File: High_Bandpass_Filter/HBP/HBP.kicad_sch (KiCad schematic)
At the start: 25 parts, among them IC2 OPA1644AIPWR

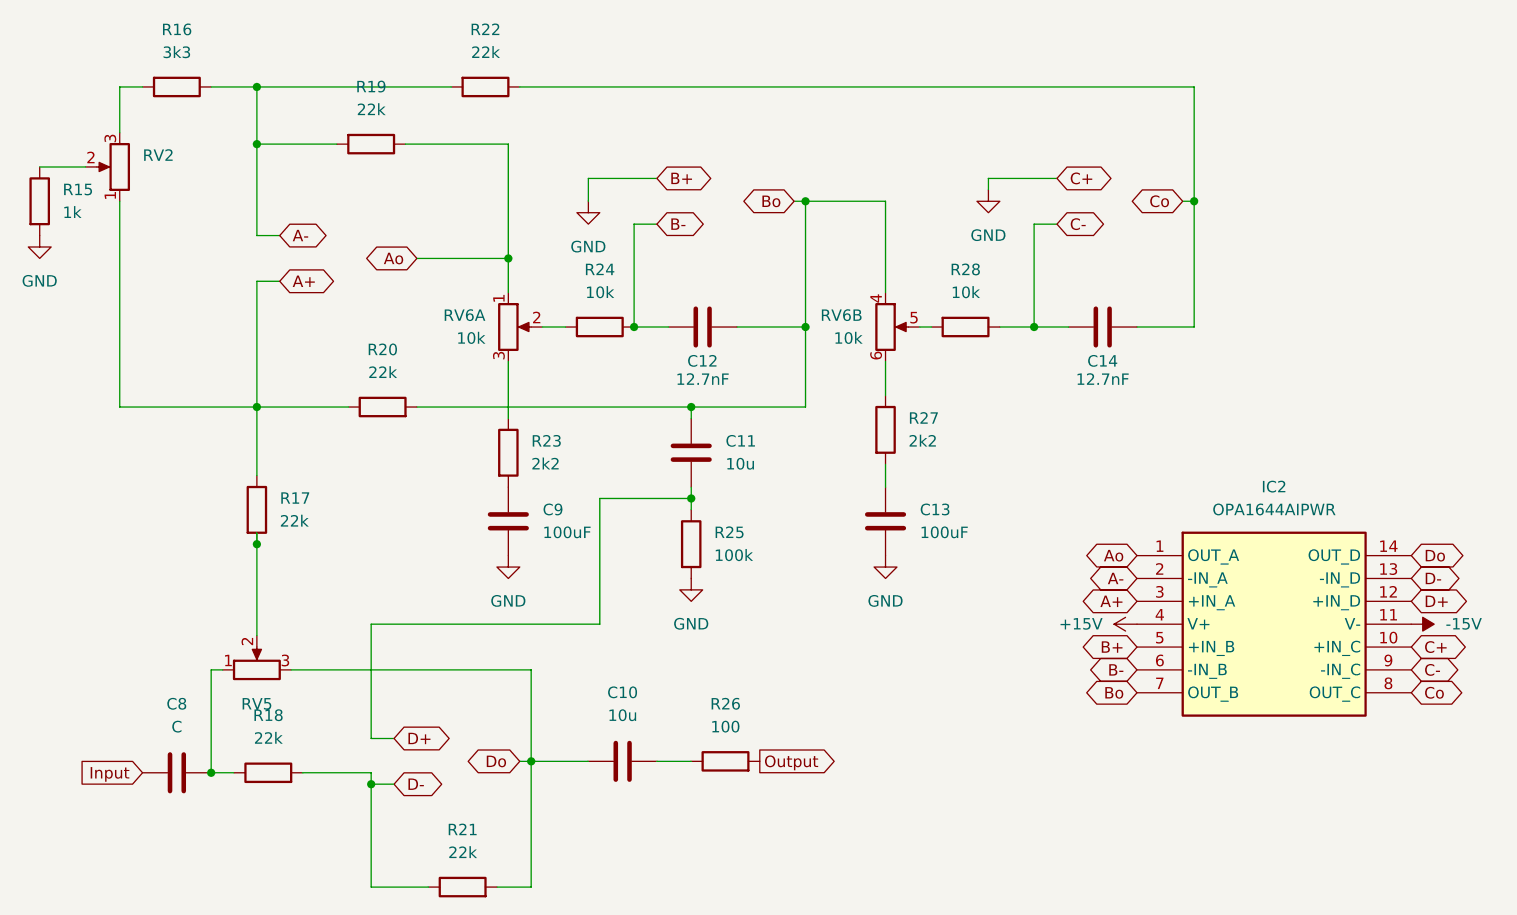
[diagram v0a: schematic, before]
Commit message: started main schematic
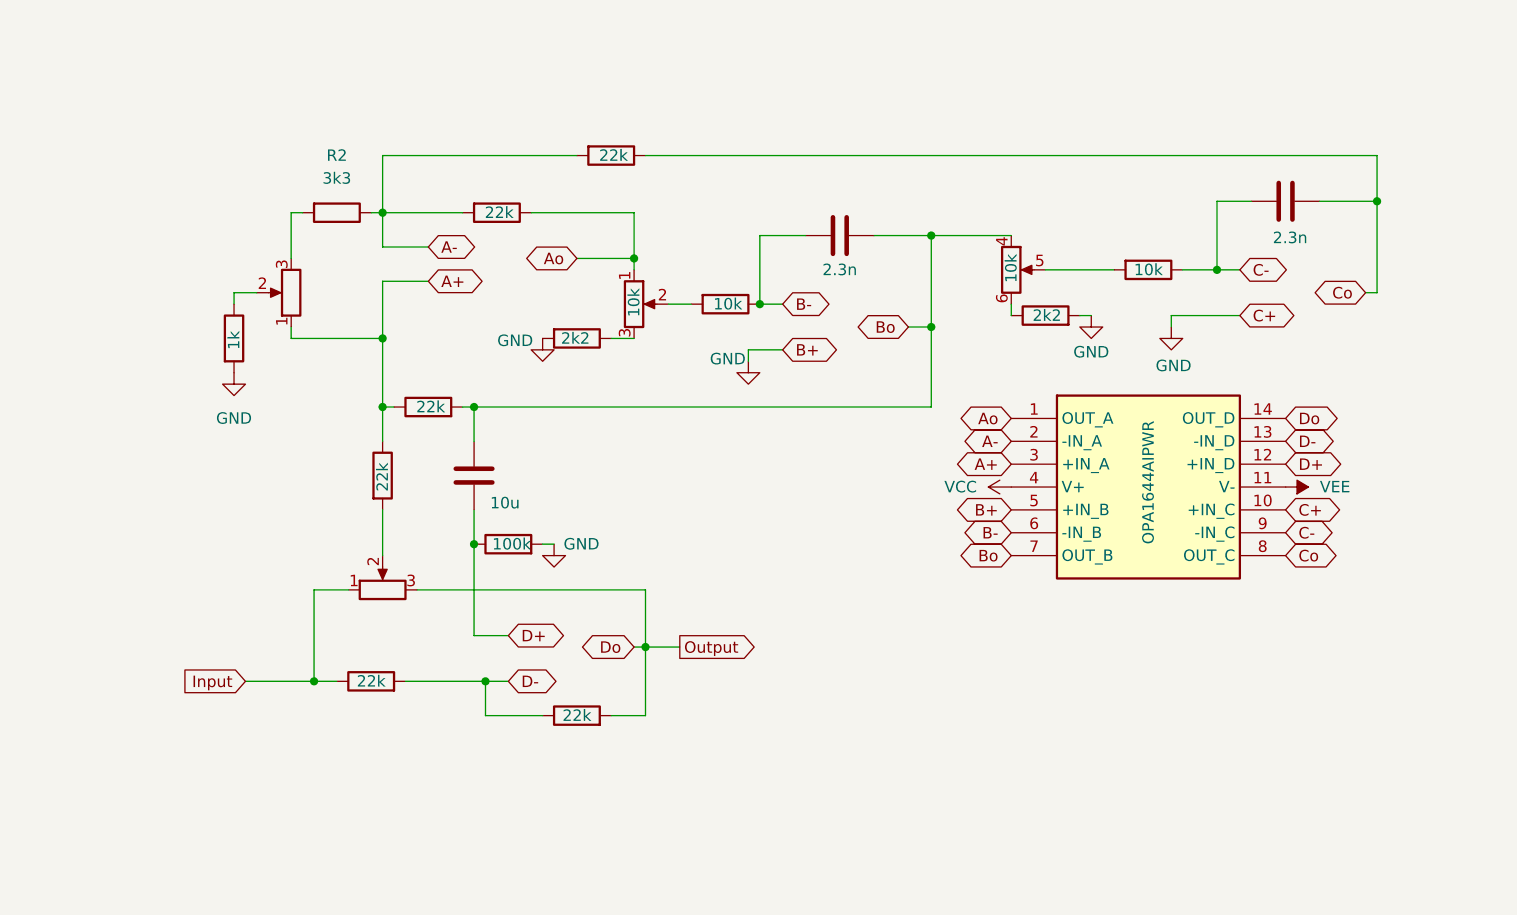
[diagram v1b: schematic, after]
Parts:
- removed C10, C11: 10u, symbol Device:C
- removed C12, C14: 12.7nF, symbol Device:C
- removed C13, C9: 100uF, symbol Device:C
- removed C8: C, symbol Device:C
- removed IC2: OPA1644AIPWR, SOP65P640X120-14N, symbol OPA1644AIPWR:OPA1644AIPWR
- removed R15: 1k, Resistor_THT:R_Axial_DIN0207_L6.3mm_D2.5mm_P10.16mm_Horizontal, symbol Device:R
- removed R16: 3k3, Resistor_THT:R_Axial_DIN0207_L6.3mm_D2.5mm_P10.16mm_Horizontal, symbol Device:R
- removed R17, R18, R19, R20, R21, R22: 22k, Resistor_THT:R_Axial_DIN0207_L6.3mm_D2.5mm_P10.16mm_Horizontal, symbol Device:R
- removed R23, R27: 2k2, Resistor_THT:R_Axial_DIN0207_L6.3mm_D2.5mm_P10.16mm_Horizontal, symbol Device:R
- removed R24, R28: 10k, Resistor_THT:R_Axial_DIN0207_L6.3mm_D2.5mm_P10.16mm_Horizontal, symbol Device:R
- removed R25: 100k, Resistor_THT:R_Axial_DIN0207_L6.3mm_D2.5mm_P10.16mm_Horizontal, symbol Device:R
- removed R26: 100, Resistor_THT:R_Axial_DIN0207_L6.3mm_D2.5mm_P10.16mm_Horizontal, symbol Device:R
- removed RV2, RV5: 10k, symbol Device:R_Potentiometer
- removed RV6: 10k, symbol Device:R_Potentiometer_Dual_Separate
- added C1, C4: 2.3n, symbol Device:C
- added C5: 10u, symbol Device:C
- added IC1: OPA1644AIPWR, SOP65P640X120-14N, symbol OPA1644AIPWR:OPA1644AIPWR
- added R1: 1k, Resistor_THT:R_Axial_DIN0207_L6.3mm_D2.5mm_P10.16mm_Horizontal, symbol Device:R
- added R10, R9: 2k2, Resistor_THT:R_Axial_DIN0207_L6.3mm_D2.5mm_P10.16mm_Horizontal, symbol Device:R
- added R11: 100k, Resistor_THT:R_Axial_DIN0207_L6.3mm_D2.5mm_P10.16mm_Horizontal, symbol Device:R
- added R12, R13, R3, R4, R5, R6: 22k, Resistor_THT:R_Axial_DIN0207_L6.3mm_D2.5mm_P10.16mm_Horizontal, symbol Device:R
- added R2: 3k3, Resistor_THT:R_Axial_DIN0207_L6.3mm_D2.5mm_P10.16mm_Horizontal, symbol Device:R
- added R7, R8: 10k, Resistor_THT:R_Axial_DIN0207_L6.3mm_D2.5mm_P10.16mm_Horizontal, symbol Device:R
- added RV1: 10k, symbol Device:R_Potentiometer_Dual_Separate
- added RV3, RV4: 10k, symbol Device:R_Potentiometer
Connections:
- net A+: now also IC1.3 (+IN_A), R5.1, R6.1, RV3.1
- net A-: now also IC1.2 (-IN_A), R2.1, R3.2, R4.2
- net Ao: now also IC1.1 (OUT_A), R3.1, RV1.1
- net B-: now also C1.1, IC1.6 (-IN_B), R7.1
- net Bo: now also C1.2, C5.2, IC1.7 (OUT_B), R5.2, RV1.4
- net C-: now also C4.1, IC1.9 (-IN_C), R8.1
- net Co: now also C4.2, IC1.8 (OUT_C), R4.1
- net D+: now also C5.1, IC1.12 (+IN_D), R11.1
- net D-: now also IC1.13 (-IN_D), R12.1, R13.2
- net Do: now also IC1.14 (OUT_D), R12.2, RV4.3
- net GND: now also IC1.10 (+IN_C), IC1.5 (+IN_B), R1.2, R10.2, R11.2, R9.2
- net Input: now also R13.1, RV4.1
- new net: R8.2, RV1.5
- new net: R10.1, RV1.6
- new net: R7.2, RV1.2
- new net: R9.1, RV1.3
- new net: R1.1, RV3.2
- new net: R2.2, RV3.3
- new net: R6.2, RV4.2
- new net VCC: IC1.4 (V+)
- new net VEE: IC1.11 (V-)
